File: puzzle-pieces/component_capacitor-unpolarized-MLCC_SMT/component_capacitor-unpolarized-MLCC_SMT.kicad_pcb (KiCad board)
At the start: 2 copper layers, 40 x 40 mm, 34 parts, among them J1 Conn_01x02_Pin, J2 Conn_01x02_Pin

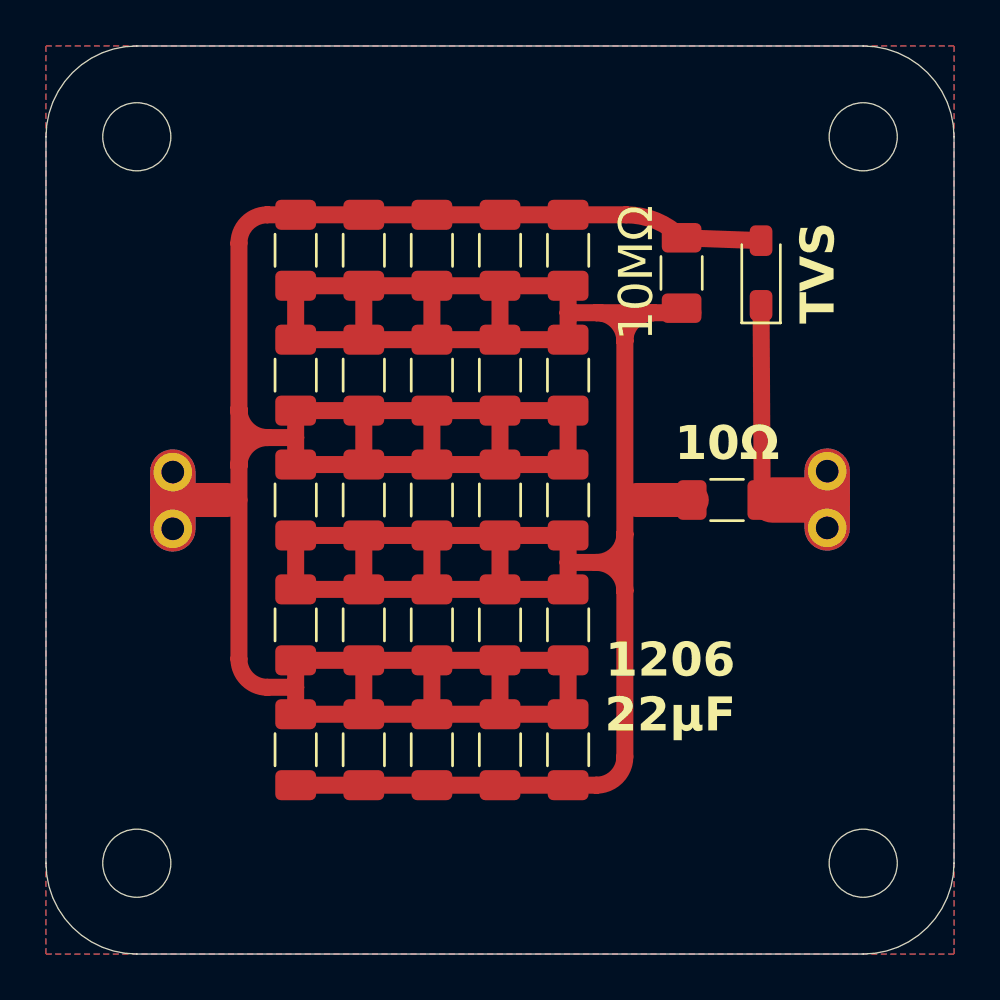
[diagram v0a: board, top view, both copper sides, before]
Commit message: rearranged images,
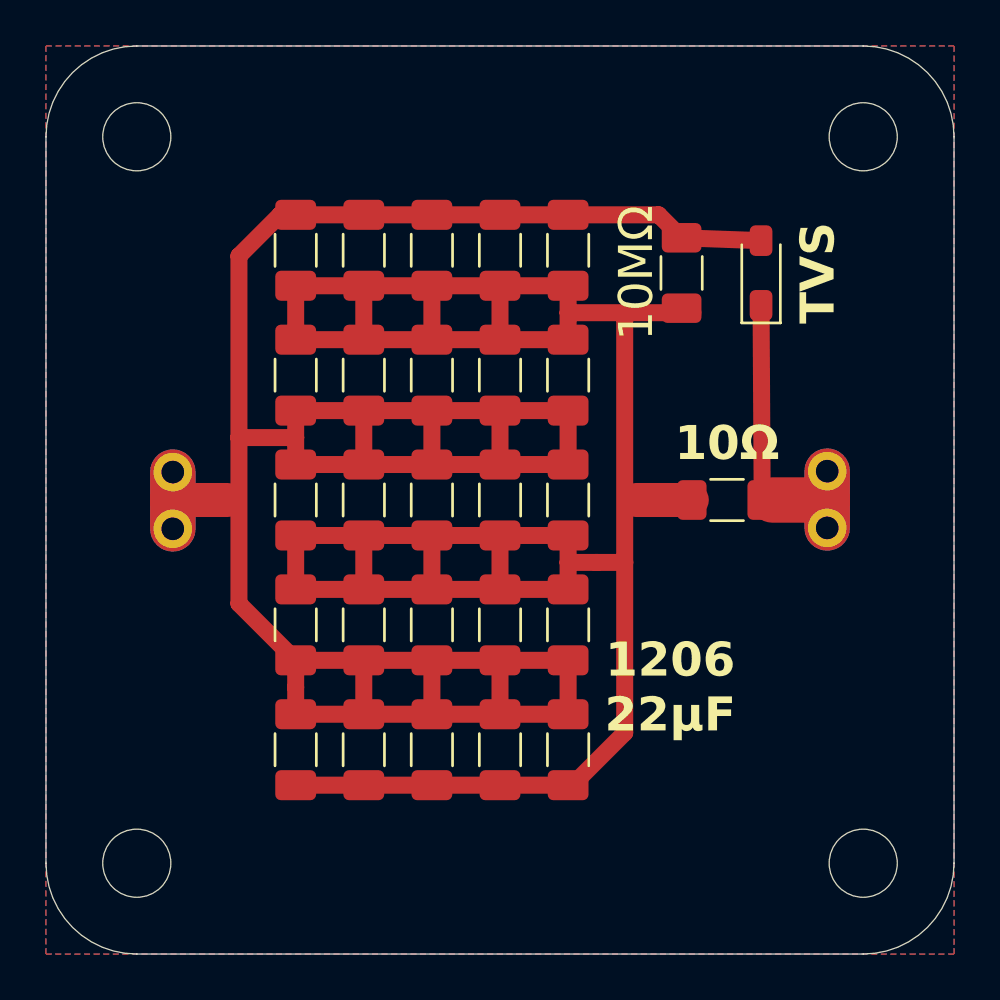
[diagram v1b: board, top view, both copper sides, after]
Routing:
- net Net-(C1-Pad1): track 122.1 -> 116.2 mm
- net Net-(D1-A2): track 129.6 -> 124.7 mm
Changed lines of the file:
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@@
 			(layer "F.Mask"
 				(type "Top Solder Mask")
-				(color "#000000E6")
+				(color "Black")
 				(thickness 0.1)
 			)
@@
 			(layer "B.Mask"
 				(type "Bottom Solder Mask")
-				(color "#000000E6")
+				(color "Black")
 				(thickness 0.1)
 			)
@@
 	)
 	(segment
-		(start 38 25.5)
-		(end 38 34)
-		(width 0.75)
-		(layer "F.Cu")
-		(net 1)
-	)
-	(segment
-		(start 38 43.8125)
-		(end 38 36.5)
+		(start 35.6875 45.0625)
+		(end 35.5 45.0625)
 		(width 0.75)
 		(layer "F.Cu")
@@
 	)
 	(segment
-		(start 26.5 23.0625)
-		(end 26.5 25.4375)
+		(start 38 24.25)
+		(end 35.5 24.25)
 		(width 0.75)
 		(layer "F.Cu")
@@
 	)
 	(segment
-		(start 39.25 24.25)
-		(end 41 24.25)
+		(start 26.5 23.0625)
+		(end 26.5 25.4375)
 		(width 0.75)
 		(layer "F.Cu")
@@
 	)
 	(segment
+		(start 38 24.25)
+		(end 37.993353 24.256647)
+		(width 0.75)
+		(layer "F.Cu")
+		(net 1)
+	)
+	(segment
+		(start 38 24.25)
+		(end 41 24.25)
+		(width 0.75)
+		(layer "F.Cu")
+		(net 1)
+	)
+	(segment
 		(start 23.5 36.4375)
 		(end 35.5 36.4375)
@@
 	)
 	(segment
-		(start 38 34)
-		(end 38 36.5)
+		(start 36.75 35.25)
+		(end 38 35.25)
 		(width 0.75)
 		(layer "F.Cu")
@@
 	)
 	(segment
-		(start 36.75 45.0625)
-		(end 35.5 45.0625)
+		(start 37.993353 42.756647)
+		(end 35.6875 45.0625)
 		(width 0.75)
 		(layer "F.Cu")
@@
 	)
 	(segment
+		(start 37.993353 24.256647)
+		(end 37.993353 42.756647)
+		(width 0.75)
+		(layer "F.Cu")
+		(net 1)
+	)
+	(segment
 		(start 35.5 25.4375)
 		(end 35.5 24.25)
@@
 	)
 	(segment
-		(start 36.75 24.25)
-		(end 39.25 24.25)
-		(width 0.75)
-		(layer "F.Cu")
-		(net 1)
-	)
-	(segment
 		(start 23.5 23.0625)
 		(end 35.5 23.0625)
@@
 	)
 	(segment
-		(start 36.75 24.25)
-		(end 35.5 24.25)
-		(width 0.75)
-		(layer "F.Cu")
-		(net 1)
-	)
-	(arc
-		(start 39.25 24.25)
-		(mid 38.366116 24.616116)
-		(end 38 25.5)
-		(width 0.75)
-		(layer "F.Cu")
-		(net 1)
-	)
-	(arc
-		(start 38 36.5)
-		(mid 37.633883 35.616116)
-		(end 36.75 35.25)
-		(width 0.75)
-		(layer "F.Cu")
-		(net 1)
-	)
-	(arc
-		(start 38 25.5)
-		(mid 37.633883 24.616116)
-		(end 36.75 24.25)
-		(width 0.75)
-		(layer "F.Cu")
-		(net 1)
-	)
-	(arc
-		(start 36.75 35.25)
-		(mid 37.633883 34.883883)
-		(end 38 34)
-		(width 0.75)
-		(layer "F.Cu")
-		(net 1)
-	)
-	(arc
-		(start 38 43.8125)
-		(mid 37.633883 44.696383)
-		(end 36.75 45.0625)
-		(width 0.75)
-		(layer "F.Cu")
-		(net 1)
-	)
-	(segment
-		(start 22.25 19.9375)
-		(end 23.5 19.9375)
-		(width 0.75)
-		(layer "F.Cu")
-		(net 2)
-	)
-	(segment
 		(start 18.0875 33.77)
 		(end 18.0875 32.5)
@@
 	)
 	(segment
-		(start 35.5 30.9375)
-		(end 35.5 28.5625)
+		(start 21 21.75)
+		(end 21 29.75)
+		(width 0.75)
+		(layer "F.Cu")
+		(net 2)
+	)
+	(segment
+		(start 21 29.75)
+		(end 23.5 29.75)
 		(width 0.75)
 		(layer "F.Cu")
@@
 	)
 	(segment
-		(start 21 21.1875)
-		(end 21 28.5)
+		(start 35.5 30.9375)
+		(end 35.5 28.5625)
 		(width 0.75)
 		(layer "F.Cu")
@@
 	)
 	(segment
-		(start 21 32.5)
-		(end 21 39.5)
+		(start 40.5 20.95)
+		(end 39.4875 19.9375)
 		(width 0.75)
 		(layer "F.Cu")
@@
 	)
 	(segment
-		(start 22.25 40.75)
-		(end 23.5 40.75)
+		(start 39.4875 19.9375)
+		(end 35.5 19.9375)
 		(width 0.75)
 		(layer "F.Cu")
@@
 	)
 	(segment
-		(start 38.055628 19.9375)
-		(end 35.5 19.9375)
-		(width 0.75)
-		(layer "F.Cu")
-		(net 2)
-	)
-	(segment
 		(start 35.5 19.9375)
 		(end 23.5 19.9375)
@@
 	)
 	(segment
-		(start 22.25 29.75)
-		(end 23.5 29.75)
-		(width 0.75)
-		(layer "F.Cu")
-		(net 2)
-	)
-	(segment
-		(start 21 31)
-		(end 21 28.5)
-		(width 0.75)
-		(layer "F.Cu")
-		(net 2)
-	)
-	(segment
 		(start 23.5 28.5625)
 		(end 35.5 28.5625)
@@
 	)
 	(segment
-		(start 21 31)
-		(end 21 32.5)
+		(start 23.5 39.5625)
+		(end 21 37.0625)
 		(width 0.75)
 		(layer "F.Cu")
@@
 	)
 	(segment
-		(start 32.5 39.5625)
-		(end 32.5 41.9375)
+		(start 21 37.0625)
+		(end 21 29.75)
 		(width 0.75)
 		(layer "F.Cu")
@@
 	)
 	(segment
-		(start 18.0875 32.5)
-		(end 20.5 32.5)
-		(width 1.5)
-		(layer "F.Cu")
-		(net 2)
-	)
-	(arc
-		(start 22.25 29.75)
-		(mid 21.366116 30.116116)
-		(end 21 31)
-		(width 0.75)
-		(layer "F.Cu")
-		(net 2)
-	)
-	(arc
-		(start 21 39.5)
-		(mid 21.366116 40.383883)
-		(end 22.25 40.75)
+		(start 32.5 39.5625)
+		(end 32.5 41.9375)
 		(width 0.75)
 		(layer "F.Cu")
 		(net 2)
 	)
-	(arc
-		(start 22.25 19.9375)
-		(mid 21.366116 20.303616)
-		(end 21 21.1875)
+	(segment
+		(start 23.5 19.9375)
+		(end 22.8125 19.9375)
 		(width 0.75)
 		(layer "F.Cu")
 		(net 2)
 	)
-	(arc
-		(start 21 28.5)
-		(mid 21.366116 29.383883)
-		(end 22.25 29.75)
+	(segment
+		(start 22.8125 19.9375)
+		(end 21 21.75)
 		(width 0.75)
 		(layer "F.Cu")
 		(net 2)
 	)
-	(arc
-		(start 40.5 20.95)
-		(mid 39.378506 20.200637)
-		(end 38.055628 19.9375)
-		(width 0.75)
+	(segment
+		(start 18.0875 32.5)
+		(end 20.5 32.5)
+		(width 1.5)
 		(layer "F.Cu")
 		(net 2)
